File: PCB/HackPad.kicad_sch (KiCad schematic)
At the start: 7 parts, among them SW1 SW_Push, SW2 SW_Push, SW3 SW_Push, SW4 SW_Push, U1 XIAO-RP2040-DIP

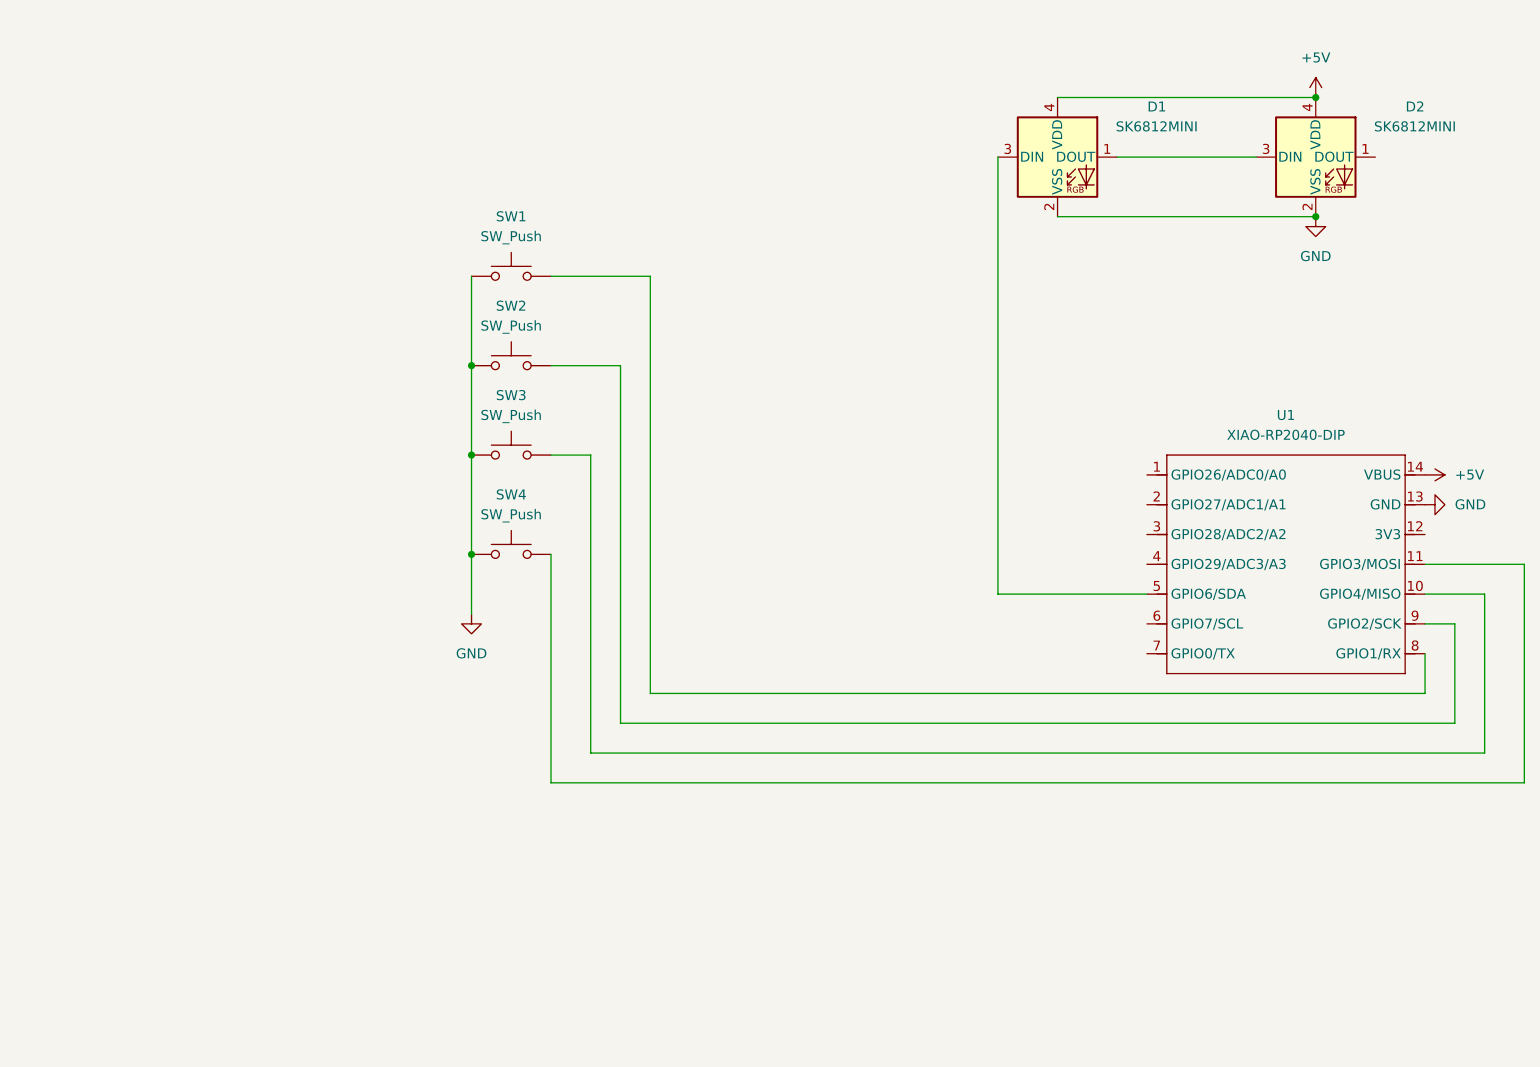
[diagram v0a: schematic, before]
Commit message: Add files via upload
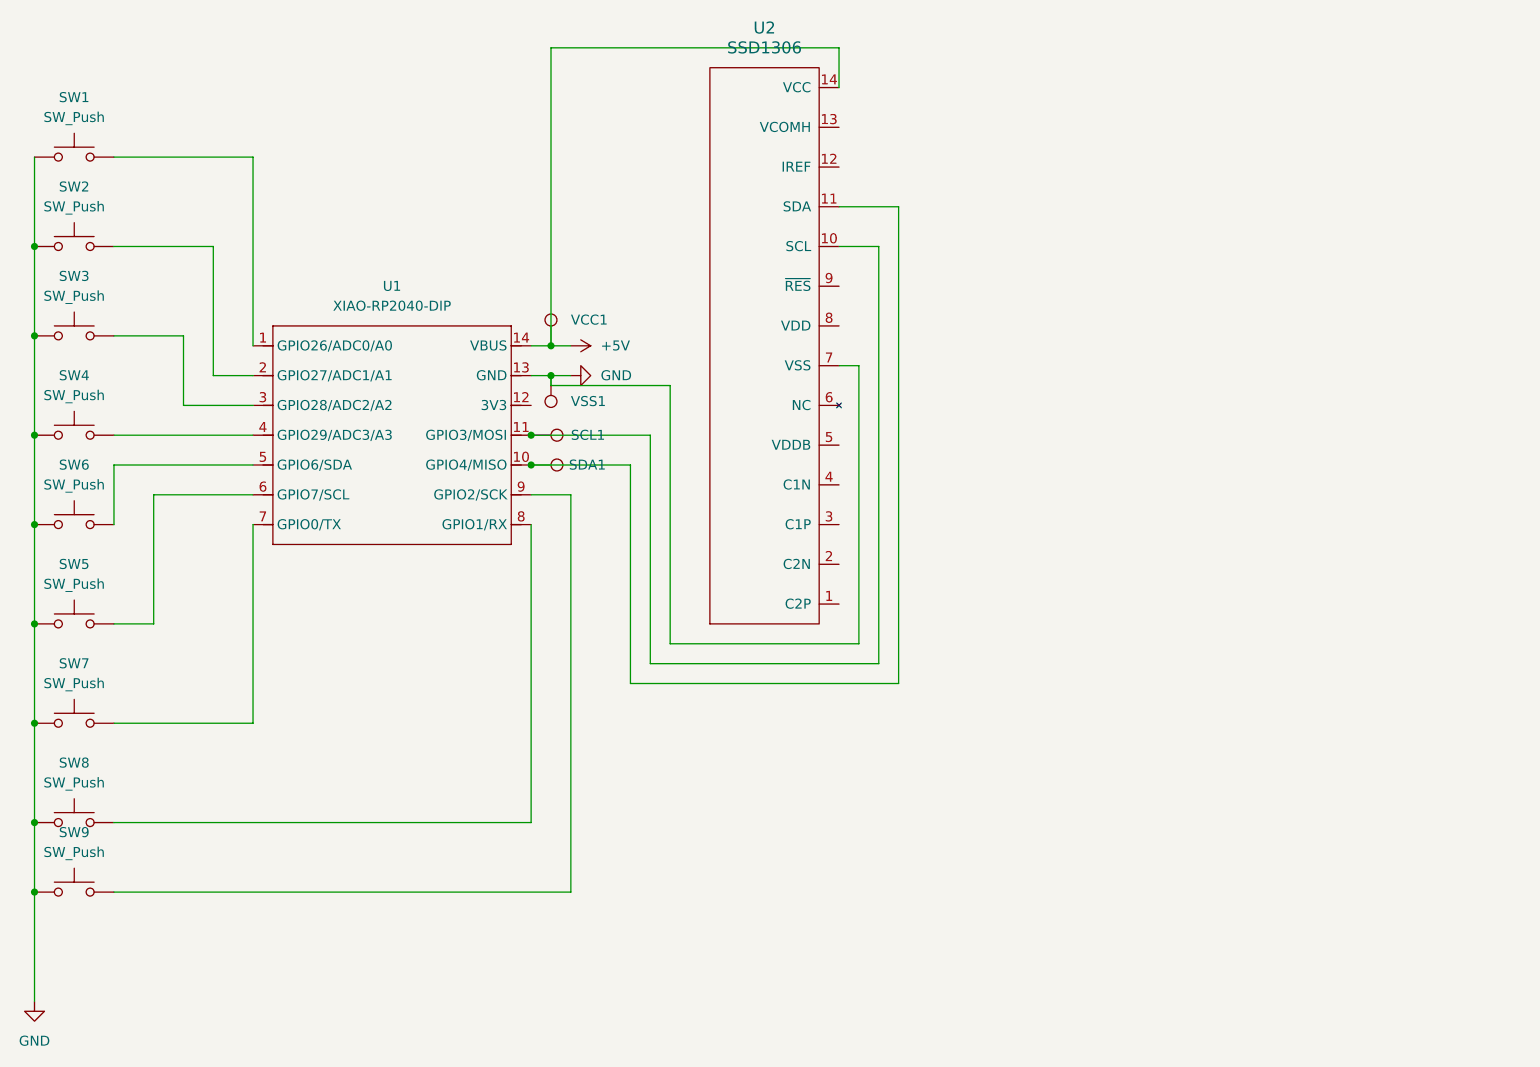
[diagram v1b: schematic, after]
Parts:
- removed D1, D2: SK6812MINI, LED_SMD:LED_SK6812MINI_PLCC4_3.5x3.5mm_P1.75mm, symbol LED:SK6812MINI
- added SCL1, SDA1, VCC1, VSS1: TestPoint, TestPoint:TestPoint_Pad_D2.0mm, symbol Connector:TestPoint
- added SW5, SW6, SW7, SW8, SW9: SW_Push, Button_Switch_Keyboard:SW_Cherry_MX_1.00u_PCB, symbol Switch:SW_Push
- added U2: SSD1306, symbol OLED:SSD1306
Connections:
- net +5V: now also U2.14 (VCC), VCC1.1
- net GND: now also SW1.2, SW2.2, SW3.2, SW4.2, SW5.2, SW6.2, SW7.2, SW8.2, SW9.2, U2.7 (VSS), VSS1.1; no longer SW1.1, SW2.1, SW3.1, SW4.1
- net at U1.8 (GPIO1/RX): now also SW8.1; no longer SW1.2
- net at U1.11 (GPIO3/MOSI): now also SCL1.1, U2.10 (SCL); no longer SW4.2
- net at U1.9 (GPIO2/SCK): now also SW9.1; no longer SW2.2
- net at U1.5 (GPIO6/SDA): now also SW6.1
- net at U1.10 (GPIO4/MISO): now also SDA1.1, U2.11 (SDA); no longer SW3.2
- net at U1.1 (GPIO26/ADC0/A0): now also SW1.1
- net at U1.2 (GPIO27/ADC1/A1): now also SW2.1
- net at U1.3 (GPIO28/ADC2/A2): now also SW3.1
- net at U1.4 (GPIO29/ADC3/A3): now also SW4.1
- net at U1.6 (GPIO7/SCL): now also SW5.1
- net at U1.7 (GPIO0/TX): now also SW7.1
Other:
- moved on the sheet: SW1, SW2, SW3, SW4, U1
